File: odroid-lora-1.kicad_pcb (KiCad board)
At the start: 2 copper layers, 48.5 x 67 mm, 8 parts, among them J1 ODROID_2x12_GPIO, J2 RASPPI_2x20_GPIO, J3 M0, J4 M1

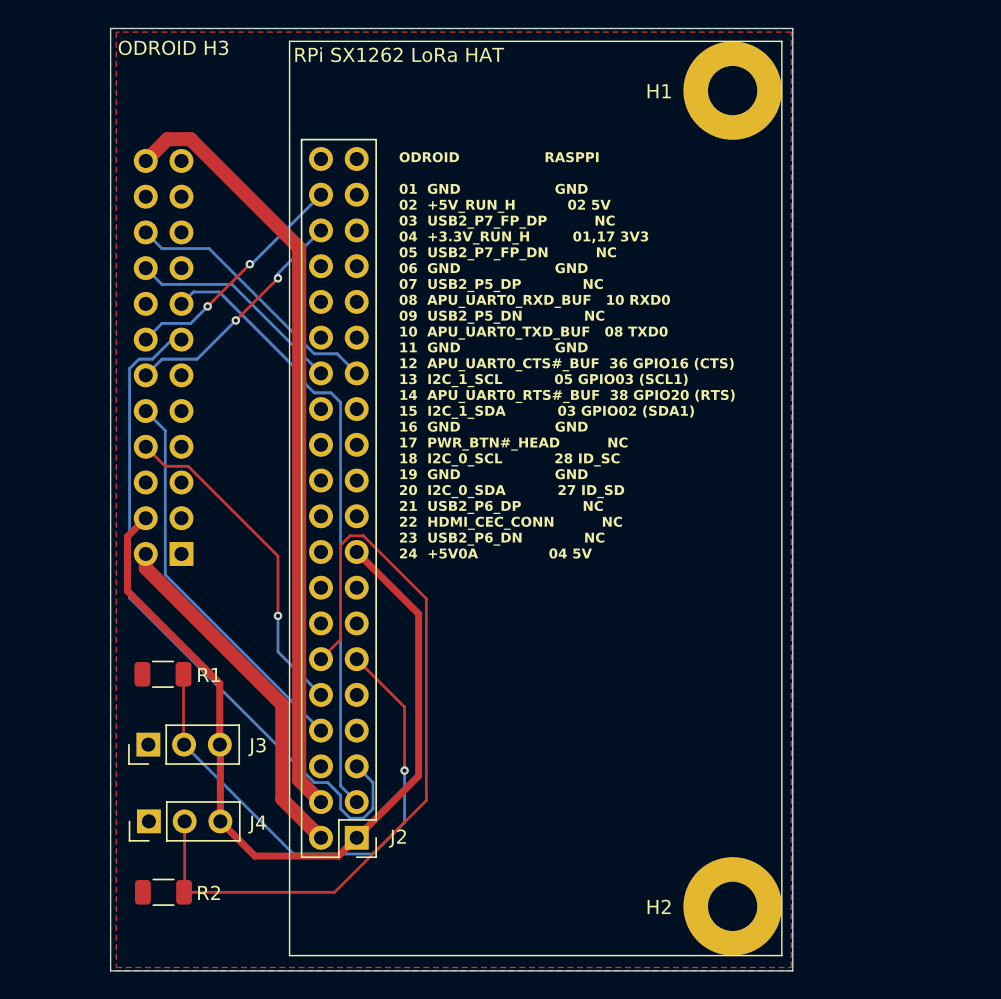
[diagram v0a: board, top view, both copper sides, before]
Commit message: add fuses
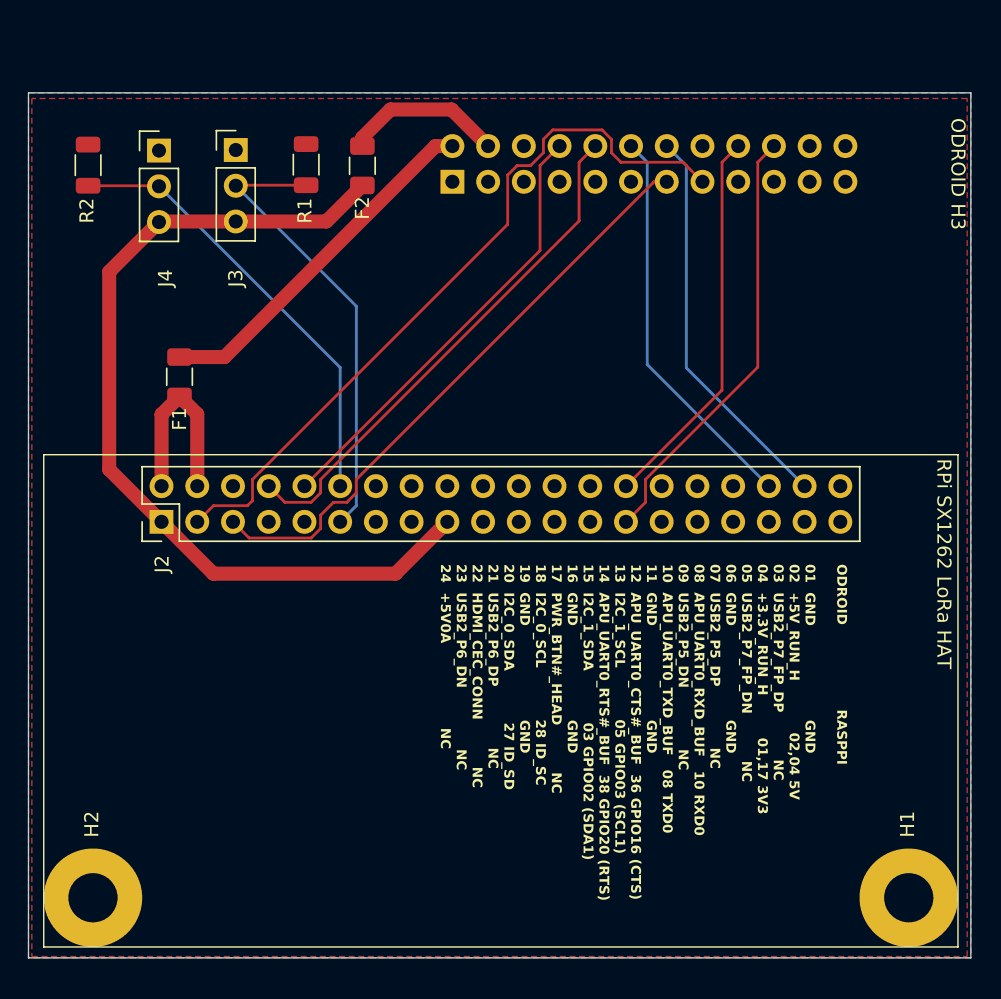
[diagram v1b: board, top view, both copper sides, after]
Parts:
- added F1: Fuse_2A, Fuse:Fuse_1206_3216Metric, F.Cu at (185.0, 111.0)
- added F2: Fuse_2A, Fuse:Fuse_1206_3216Metric, F.Cu at (198.0, 96.0)
- H1, H2: value MountingHole_SX1268 -> MOUNT_SX1268
- J1: value ODROID_2x12_GPIO -> ODROID_2x12_SOCKET
- J2: value RASPPI_2x20_GPIO -> RASPPI_2x20_HEADER
- J3: value M0 -> Mode0
- J4: value M1 -> Mode1
- R1, R2: value 47K -> 51K
- moved H1 58.7 mm to (236.8, 148.0), turned to 180 degrees
- moved R2 52.0 mm to (178.5, 96.0), turned to 90 degrees
- moved J4 47.7 mm to (183.5, 94.9), turned to 0 degrees
- moved H2 45.5 mm to (178.8, 148.0), turned to 180 degrees
- moved J3 42.7 mm to (189.0, 94.9), turned to 0 degrees
- moved R1 37.6 mm to (194.0, 95.9), turned to 90 degrees
- moved J1 32.7 mm to (204.4, 97.1), turned to -90 degrees
- moved J2 26.4 mm to (183.7, 121.3), turned to 90 degrees
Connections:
- net +3V3 renamed /3V_RUN_H
- net GND renamed /GND
- net Net-(J1-Pin_10) renamed /UART0_TXD
- net Net-(J1-Pin_12) renamed /UART0_CTS
- net Net-(J1-Pin_13) renamed /I2C1_SCL
- net Net-(J1-Pin_14) renamed /UART0_RTS
- net Net-(J1-Pin_15) renamed /I2C1_SDA
- net Net-(J1-Pin_18) renamed /I2C0_SCL
- net Net-(J1-Pin_20) renamed /I2C0_SDA
- net Net-(J1-Pin_8) renamed /UART0_RXD
- net Net-(J2-Pin_11) renamed /GPIO_M0
- net Net-(J2-Pin_12) renamed /GPIO_M1
- J1 pad 2: +5VA -> /5V_RUN_H
- J1 pad 24: +5VB -> unconnected-(J1-Pin_24-Pad24)
- J2 pad 2: +5VA -> /5V_RUN_H
- J2 pad 4: +5VB -> /5V_RUN_H
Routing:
- net +5VB: track 54.8 -> 0.00 mm
- net /5V_RUN_H: track 0.00 -> 39.4 mm
- net +5VA: track 25.3 -> 0.00 mm
- net /GPIO_M1: track 56.2 -> 31.7 mm
- net /3V_RUN_H: track 60.1 -> 74.7 mm
- net /I2C0_SDA: track 19.2 -> 31.1 mm
- net /I2C0_SCL: track 15.6 -> 27.5 mm
- net /UART0_RTS: track 16.7 -> 28.2 mm, vias 2 -> 0
- net /UART0_CTS: track 16.9 -> 28.2 mm, vias 2 -> 0
- net /UART0_TXD: track 27.9 -> 37.2 mm
- net /I2C1_SDA: track 44.1 -> 53.0 mm
- net /UART0_RXD: track 23.8 -> 31.7 mm, vias 1 -> 0
- net /I2C1_SCL: track 49.0 -> 42.9 mm
- net /GPIO_M0: track 37.9 -> 32.9 mm, vias 1 -> 0
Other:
- board size 48.5 x 67 mm -> 67 x 61.5 mm
- board text added: "ODROID RASPPI 01 GND GND 02 +5V_RUN_H 02,04 5V 03 USB2_P7_FP_DP NC 04 +3.3V_RUN_H 01,17 3V3 05 USB2_P7_FP_DN NC 06 GND GND 07 USB2_P5_DP NC 08 APU_UART0_RXD_BUF 10 RXD0 09 USB2_P5_DN NC 10 APU_UART0_TXD_BUF 08 TXD0 11 GND GND 12 APU_UART0_CTS#_BUF 36 GPIO16 (CTS) 13 I2C_1_SCL 05 GPIO03 (SCL1) 14 APU_UART0_RTS#_BUF 38 GPIO20 (RTS) 15 I2C_1_SDA 03 GPIO02 (SDA1) 16 GND GND 17 PWR_BTN#_HEAD NC 18 I2C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"
- board text removed: "ODROID RASPPI 01 GND GND 02 +5V_RUN_H 02 5V 03 USB2_P7_FP_DP NC 04 +3.3V_RUN_H 01,17 3V3 05 USB2_P7_FP_DN NC 06 GND GND 07 USB2_P5_DP NC 08 APU_UART0_RXD_BUF 10 RXD0 09 USB2_P5_DN NC 10 APU_UART0_TXD_BUF 08 TXD0 11 GND GND 12 APU_UART0_CTS#_BUF 36 GPIO16 (CTS) 13 I2C_1_SCL 05 GPIO03 (SCL1) 14 APU_UART0_RTS#_BUF 38 GPIO20 (RTS) 15 I2C_1_SDA 03 GPIO02 (SDA1) 16 GND GND 17 PWR_BTN#_HEAD NC 18 I2C_0_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"
